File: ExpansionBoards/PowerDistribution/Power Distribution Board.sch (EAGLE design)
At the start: 27 parts, among them J1 350211-1, J10 640445-3, J11 640445-5, J12 640445-8, J13 640445-6, J14 216571-2003, J15 640445-6, J2 216571-2005, J3 216571-2004, J4 216571-2003, J5 350211-1, J6 216571-2002, J7 216571-2008, J8 640445-6, J9 640445-2, K1 AHQSS105DM2FA0G, U3 LM338T/NOPB

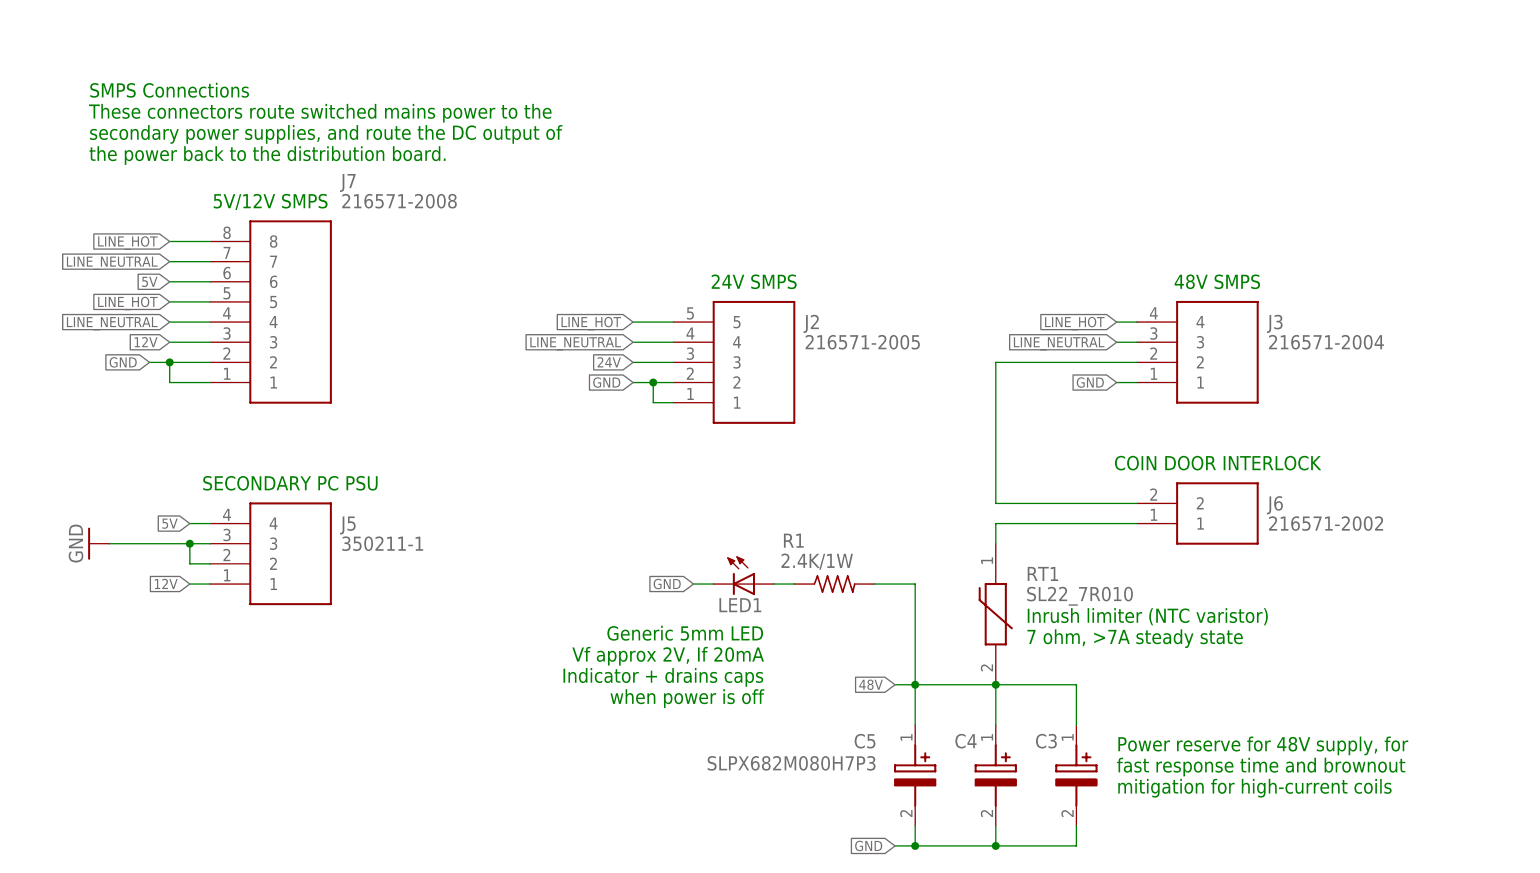
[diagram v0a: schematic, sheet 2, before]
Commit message: KL25Z adapter board updates;
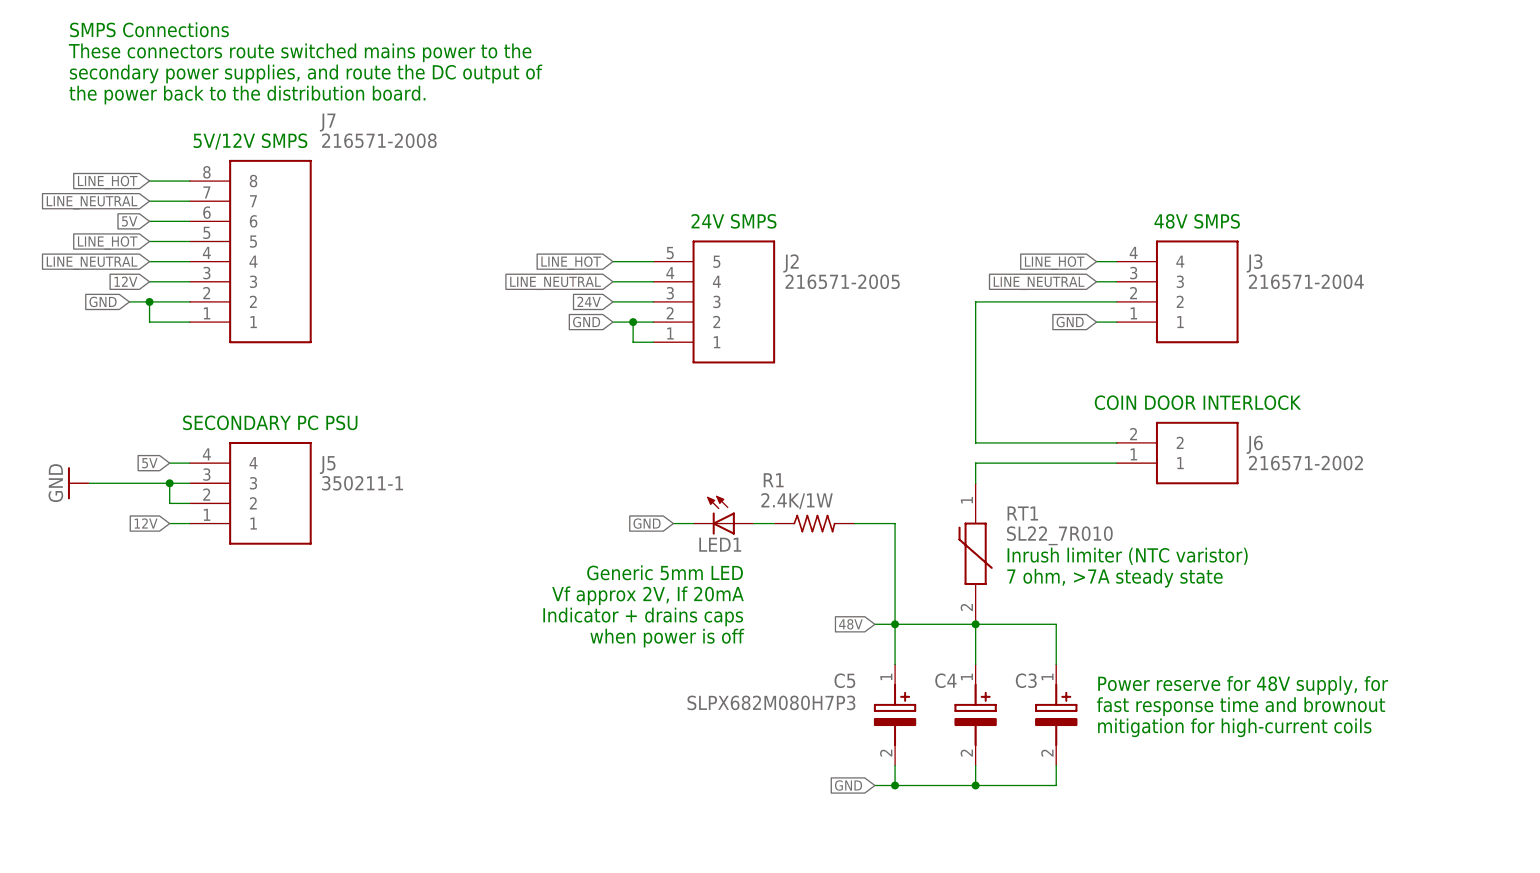
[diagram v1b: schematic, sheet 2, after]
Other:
- moved on the sheet: C3, C4, C5, J2, J3, J5, J6, J7, LED1, R1, RT1
